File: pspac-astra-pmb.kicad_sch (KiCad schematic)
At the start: 15 parts, among them J1 Conn_01x02_Socket, J2 Conn_01x01_Socket, J3 Screw_Terminal_01x03, J5 Screw_Terminal_01x01, J6 Screw_Terminal_01x01, Q1 BSC014N04LSIATMA1, U1 INA226, U5 LD1117V33

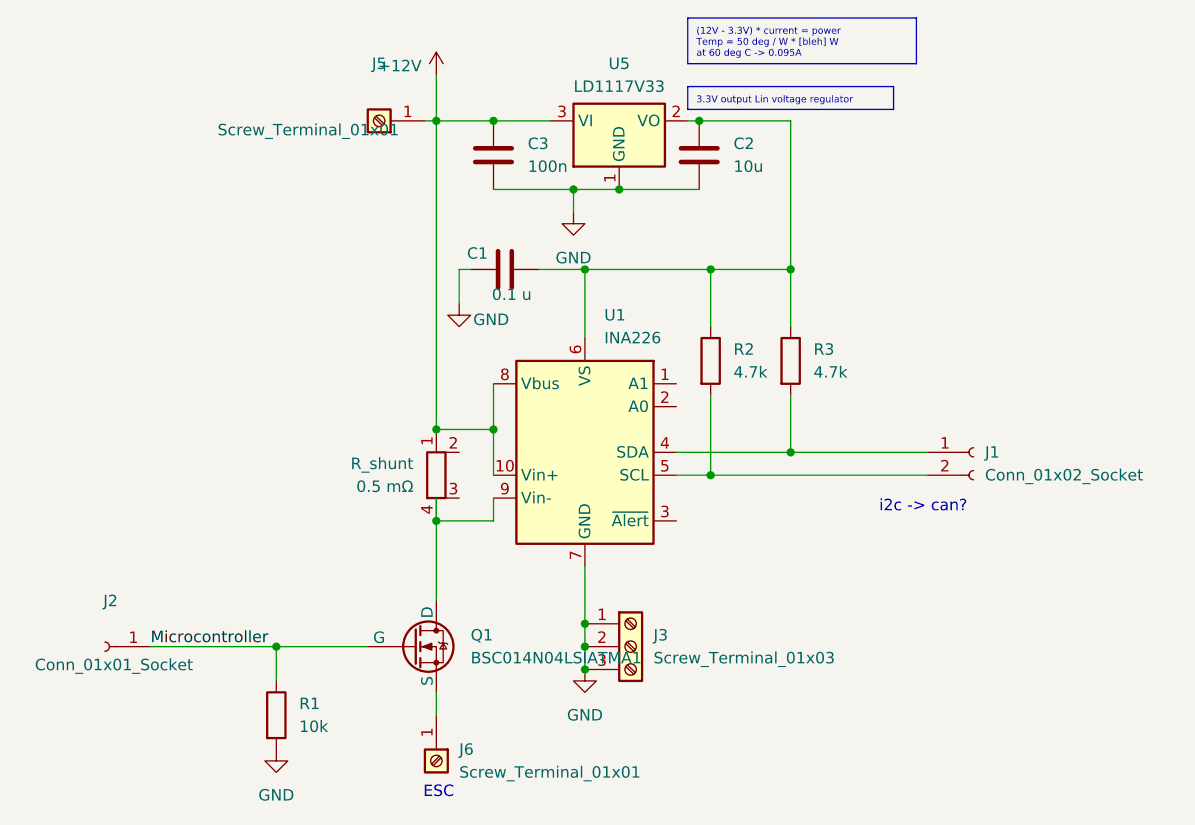
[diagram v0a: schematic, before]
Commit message: Add files via upload
shunt resistor footprint added
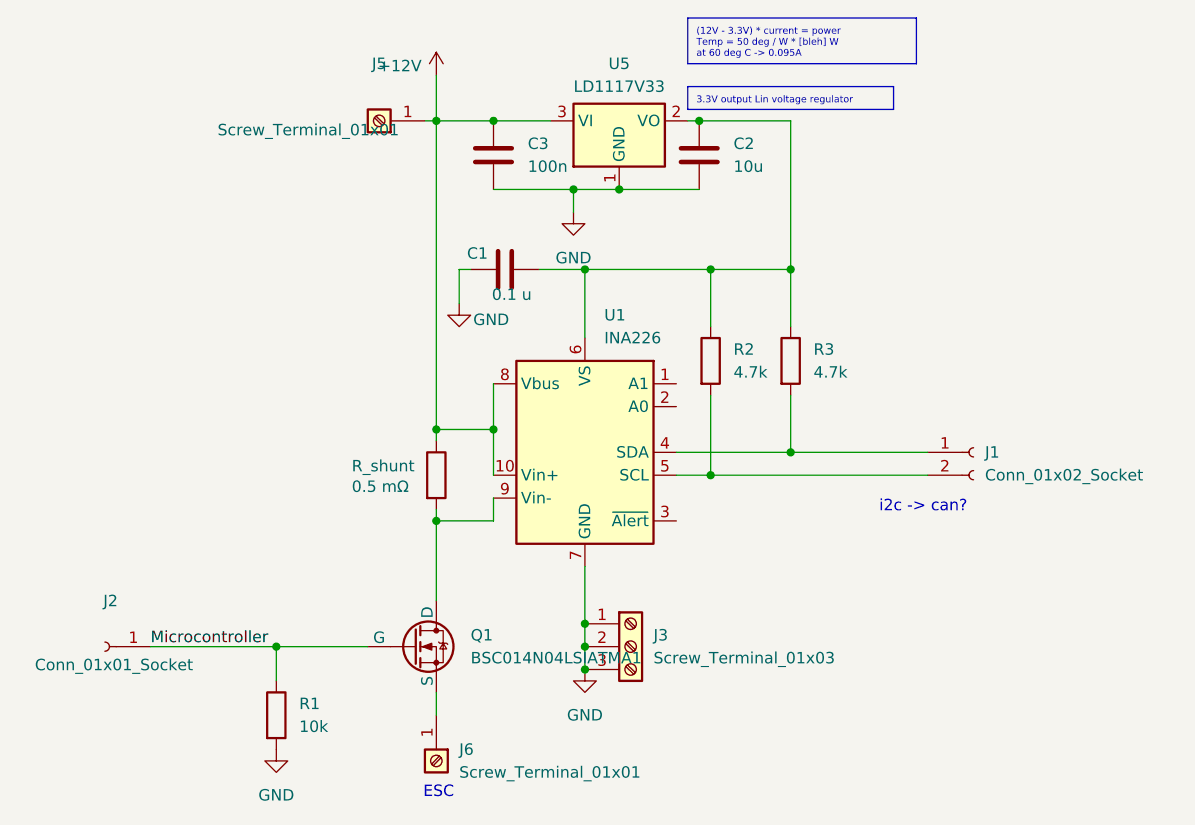
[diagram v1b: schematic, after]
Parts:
- removed R_shunt: 0.5 mΩ, symbol Device:R_Shunt
- added R_shunt: 0.5 mΩ, symbol Device:R
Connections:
- net +12V: now also R_shunt.1
- net at Q1.1 (D), U1.9 (Vin-): now also R_shunt.2
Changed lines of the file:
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@@
+	)
+	(junction
+		(at 101.6 59.69)
+		(diameter 0)
+		(color 0 0 0 0)
 	)
 	(junction
@@
 	)
 	(junction
+		(at 116.84 33.02)
+		(diameter 0)
+		(color 0 0 0 0)
+	)
+	(junction
+		(at 118.11 81.28)
+		(diameter 0)
+		(color 0 0 0 0)
+	)
+	(junction
+		(at 101.6 25.4)
+		(diameter 0)
+		(color 0 0 0 0)
+	)
+	(junction
+		(at 130.81 25.4)
+		(diameter 0)
+		(color 0 0 0 0)
+	)
+	(junction
+		(at 118.11 86.36)
+		(diameter 0)
+		(color 0 0 0 0)
+	)
+	(junction
+		(at 121.92 33.02)
+		(diameter 0)
+		(color 0 0 0 0)
+	)
+	(junction
+		(at 132.08 41.91)
+		(diameter 0)
+		(color 0 0 0 0)
+	)
+	(junction
+		(at 107.95 59.69)
+		(diameter 0)
+		(color 0 0 0 0)
+	)
+	(junction
+		(at 132.08 64.77)
+		(diameter 0)
+		(color 0 0 0 0)
+	)
+	(junction
 		(at 101.6 69.85)
 		(diameter 0)
@@
 	)
 	(junction
-		(at 116.84 33.02)
-		(diameter 0)
-		(color 0 0 0 0)
-	)
-	(junction
-		(at 118.11 81.28)
-		(diameter 0)
-		(color 0 0 0 0)
-	)
-	(junction
-		(at 101.6 25.4)
-		(diameter 0)
-		(color 0 0 0 0)
-	)
-	(junction
-		(at 130.81 25.4)
-		(diameter 0)
-		(color 0 0 0 0)
-	)
-	(junction
-		(at 101.6 59.69)
-		(diameter 0)
-		(color 0 0 0 0)
-	)
-	(junction
-		(at 118.11 86.36)
-		(diameter 0)
-		(color 0 0 0 0)
-	)
-	(junction
-		(at 121.92 33.02)
-		(diameter 0)
-		(color 0 0 0 0)
-	)
-	(junction
-		(at 132.08 41.91)
-		(diameter 0)
-		(color 0 0 0 0)
-	)
-	(junction
-		(at 107.95 59.69)
-		(diameter 0)
-		(color 0 0 0 0)
-	)
-	(junction
-		(at 132.08 64.77)
-		(diameter 0)
-		(color 0 0 0 0)
-	)
-	(junction
 		(at 83.82 83.82)
 		(diameter 0)
@@
 	(wire
 		(pts
-			(xy 101.6 67.31) (xy 101.6 69.85)
-		)
-		(stroke
-			(width 0)
-			(type default)
-		)
-	)
-	(wire
-		(pts
 			(xy 101.6 20.32) (xy 101.6 25.4)
 		)
@@
 	(wire
 		(pts
+			(xy 101.6 59.69) (xy 101.6 60.96)
+		)
+		(stroke
+			(width 0)
+			(type default)
+		)
+	)
+	(wire
+		(pts
 			(xy 130.81 25.4) (xy 140.97 25.4)
 		)
@@
 		(pts
 			(xy 107.95 33.02) (xy 116.84 33.02)
+		)
+		(stroke
+			(width 0)
+			(type default)
+		)
+	)
+	(wire
+		(pts
+			(xy 101.6 68.58) (xy 101.6 69.85)
 		)
 		(stroke
@@
 	)
 	(symbol
-		(lib_id "Device:R_Shunt")
+		(lib_id "Device:R")
 		(at 101.6 64.77 0)
 		(unit 1)
@@
 		(dnp no)
 		(property "Reference" "R_shunt"
-			(at 99.06 63.4999 0)
-			(effects
-				(font
-					(size 1.27 1.27)
-				)
-				(justify right)
+			(at 92.202 63.754 0)
+			(effects
+				(font
+					(size 1.27 1.27)
+				)
+				(justify left)
 			)
 		)
 		(property "Value" "0.5 mΩ"
-			(at 99.06 66.0399 0)
-			(effects
-				(font
-					(size 1.27 1.27)
-				)
-				(justify right)
+			(at 92.202 66.04 0)
+			(effects
+				(font
+					(size 1.27 1.27)
+				)
+				(justify left)
 			)
 		)
@@
 			)
 		)
-		(property "Datasheet" "https://fscdn.rohm.com/en/products/databook/datasheet/passive/resistor/chip_resistor/gmr-e.pdf"
+		(property "Datasheet" "~"
 			(at 101.6 64.77 0)
 			(effects
@@
 			)
 		)
-		(property "Description" "Shunt resistor with Kelvin connections"
+		(property "Description" "Resistor"
 			(at 101.6 64.77 0)
 			(effects
@@
 		(pin "1"
 		)
-		(pin "4"
-		)
 		(pin "2"
 		)
-		(pin "3"
-		)
 		(instances
